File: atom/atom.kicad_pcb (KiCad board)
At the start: 2 copper layers, 109 x 54 mm, 64 parts, among them J10 TC2030_NL, J101 MALE, J1010 MALE, J102 FEMALE, J103 MALE, J1030 MALE, J104 FEMALE, J105 MALE, J1050 MALE, J106 FEMALE, J107 MALE, J1070 MALE, J108 FEMALE, J11 STANDOFF, J111 STANDOFF, J112 STANDOFF, J113 STANDOFF, J114 STANDOFF, J12 STANDOFF, J13 STANDOFF, J14 STANDOFF, J2 FEMALE, J4 FEMALE, J6 FEMALE, J8 FEMALE, J9 DTR, Q1 2N3904, SW1 ACTION, SW2 ACTION, SW3 ACTION, SW4 ACTION, U3 ATmega328P-MU, Y1 YSX321SL

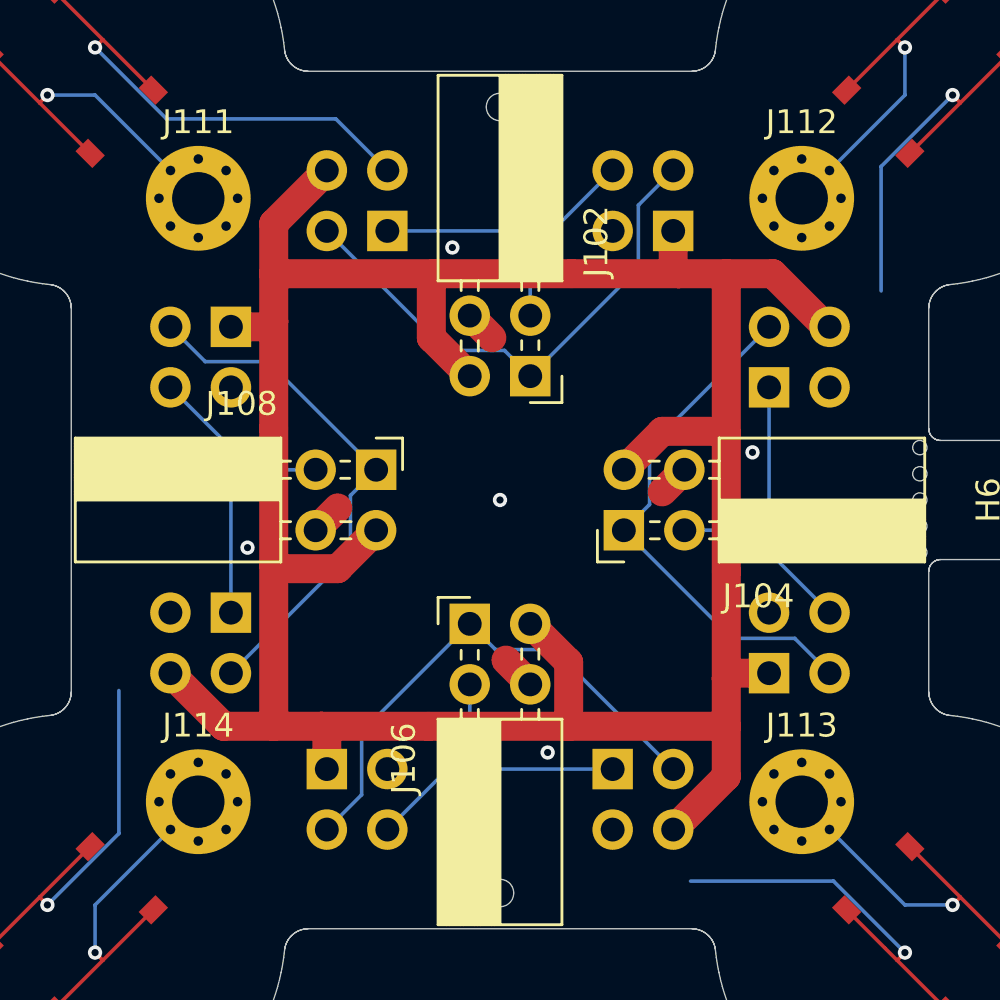
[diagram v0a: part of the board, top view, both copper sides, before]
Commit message: Reroute
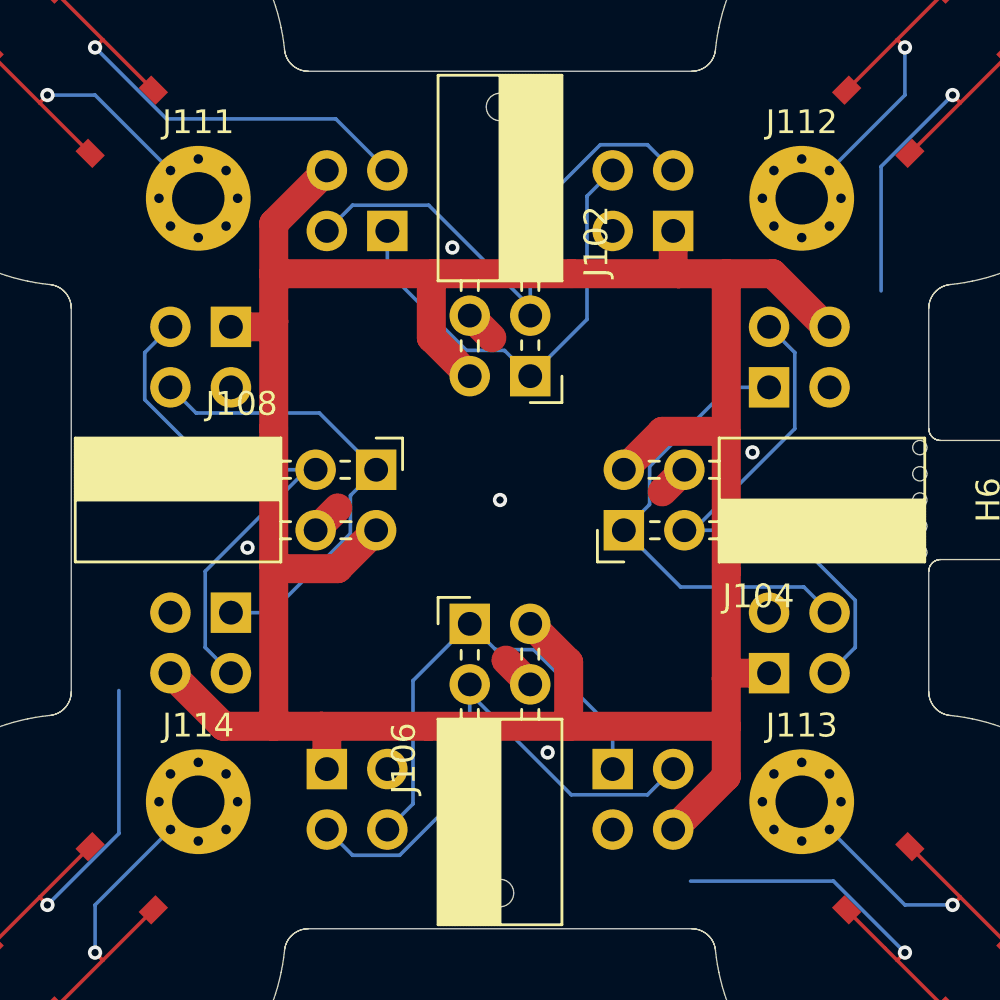
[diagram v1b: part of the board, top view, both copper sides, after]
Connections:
- J101 pad 2: Net-(J101-Pad2) -> /Upper Board/RX1T
- J101 pad 4: Net-(J101-Pad4) -> /Upper Board/TX1T
- J1010 pad 1: Net-(J101-Pad4) -> /Upper Board/TX1T
- J1010 pad 3: Net-(J101-Pad2) -> /Upper Board/RX1T
- J102 pad 1: Net-(J101-Pad2) -> /Upper Board/TX1T
- J102 pad 2: Net-(J101-Pad4) -> /Upper Board/RX1T
- J103 pad 2: Net-(J103-Pad2) -> /Upper Board/RX2T
- J103 pad 4: Net-(J103-Pad4) -> /Upper Board/TX2T
- J1030 pad 1: Net-(J103-Pad4) -> /Upper Board/TX2T
- J1030 pad 3: Net-(J103-Pad2) -> /Upper Board/RX2T
- J104 pad 1: Net-(J103-Pad2) -> /Upper Board/TX2T
- J104 pad 2: Net-(J103-Pad4) -> /Upper Board/RX2T
- J105 pad 2: Net-(J105-Pad2) -> /Upper Board/RX3T
- J105 pad 4: Net-(J105-Pad4) -> /Upper Board/TX3T
- J1050 pad 1: Net-(J105-Pad4) -> /Upper Board/TX3T
- J1050 pad 3: Net-(J105-Pad2) -> /Upper Board/RX3T
- J106 pad 1: Net-(J105-Pad2) -> /Upper Board/TX3T
- J106 pad 2: Net-(J105-Pad4) -> /Upper Board/RX3T
- J107 pad 2: Net-(J107-Pad2) -> /Upper Board/RX4T
- J107 pad 4: Net-(J107-Pad4) -> /Upper Board/TX4T
- J1070 pad 1: Net-(J107-Pad4) -> /Upper Board/TX4T
- J1070 pad 3: Net-(J107-Pad2) -> /Upper Board/RX4T
- J108 pad 1: Net-(J107-Pad2) -> /Upper Board/TX4T
- J108 pad 2: Net-(J107-Pad4) -> /Upper Board/RX4T
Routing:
- net /Upper Board/RX1T: track 0.00 -> 23.0 mm
- net /Upper Board/RX3T: track 0.00 -> 23.0 mm
- net /Upper Board/RX4T: track 0.00 -> 23.0 mm
- net /Upper Board/RX2T: track 0.00 -> 23.0 mm
- net Net-(J105-Pad2): track 22.2 -> 0.00 mm
- net Net-(J103-Pad2): track 22.2 -> 0.00 mm
- net Net-(J101-Pad2): track 22.2 -> 0.00 mm
- net Net-(J107-Pad2): track 22.2 -> 0.00 mm
- net /Upper Board/TX4T: track 0.00 -> 19.6 mm
- net /Upper Board/TX3T: track 0.00 -> 19.6 mm
- net /Upper Board/TX1T: track 0.00 -> 19.6 mm
- net /Upper Board/TX2T: track 0.00 -> 19.6 mm
- net Net-(J101-Pad4): track 14.0 -> 0.00 mm
- net Net-(J103-Pad4): track 14.0 -> 0.00 mm
- net Net-(J107-Pad4): track 13.9 -> 0.00 mm
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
